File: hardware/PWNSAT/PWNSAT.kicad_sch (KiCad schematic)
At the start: 0 parts

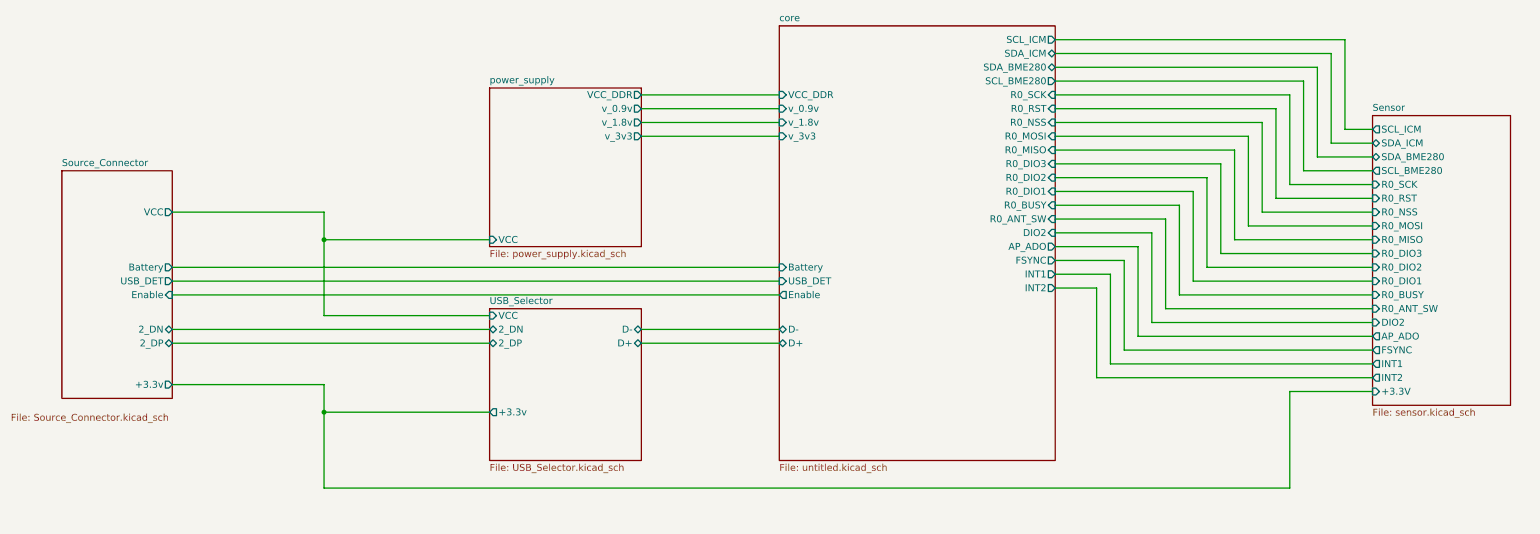
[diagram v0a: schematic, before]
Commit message: feat(Hw):floorplans_updated
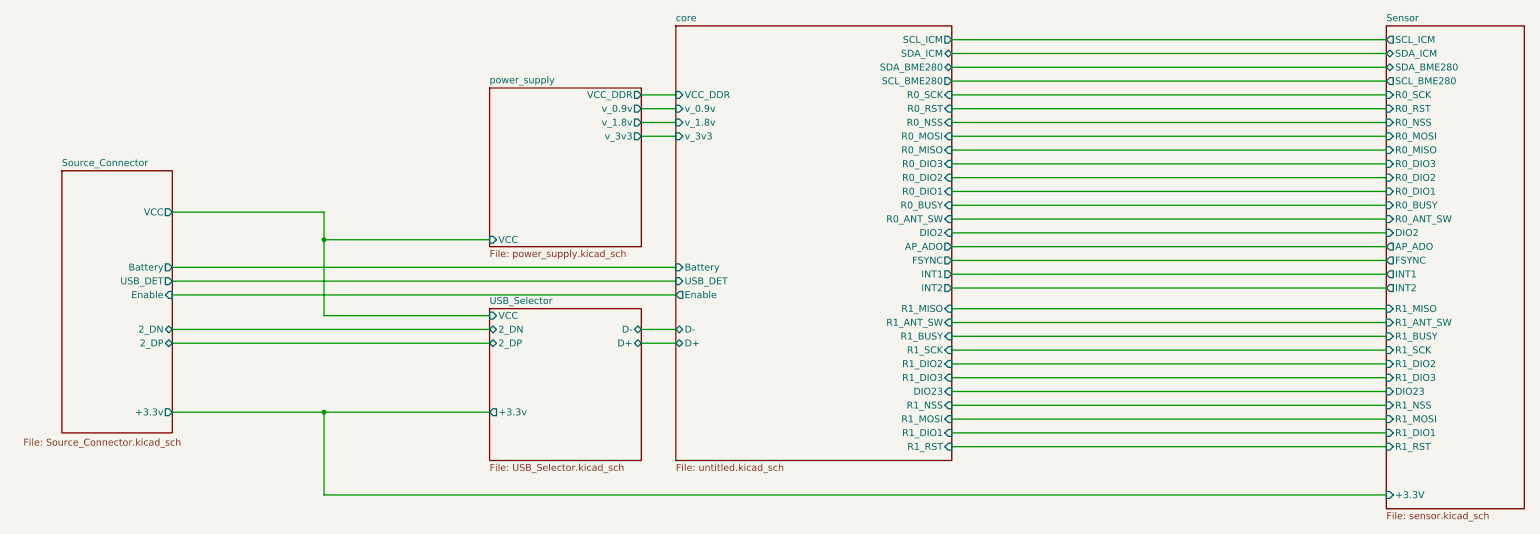
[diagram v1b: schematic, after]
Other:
- sheet Sensor ports: added DIO23, R1_ANT_SW, R1_BUSY, R1_DIO1, R1_DIO2, R1_DIO3, R1_MISO, R1_MOSI, R1_NSS, R1_RST, R1_SCK; removed none
- sheet core ports: added DIO23, R1_ANT_SW, R1_BUSY, R1_DIO1, R1_DIO2, R1_DIO3, R1_MISO, R1_MOSI, R1_NSS, R1_RST, R1_SCK; removed none
